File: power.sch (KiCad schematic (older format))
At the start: 44 parts, among them CON1 BARREL_JACK, J1 JMP, U2 WM8778-units, U3 AP3211, U4 AZ1117C, U5 TC1185

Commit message: ksch: add stuff that isn't on soldered prototype yet
this hopefully completes the rev. A schematics
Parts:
- C201: renamed from C1; footprint (none) -> Capacitors_SMD:C_0805_HandSoldering
- C202: renamed from C2; footprint (none) -> Capacitors_SMD:C_0805_HandSoldering
- C203: renamed from C3; footprint (none) -> Capacitors_SMD:C_0805_HandSoldering
- C204: renamed from C4; footprint (none) -> Capacitors_SMD:C_0805_HandSoldering
- C205: renamed from C5; footprint (none) -> Capacitors_SMD:C_0805_HandSoldering
- C206: renamed from C6; footprint (none) -> Capacitors_SMD:C_0805_HandSoldering
- C207: renamed from C7; footprint (none) -> Capacitors_SMD:C_0805_HandSoldering
- C208: renamed from C8; footprint (none) -> Capacitors_SMD:C_0805_HandSoldering
- C209: renamed from C9; footprint (none) -> Capacitors_SMD:C_0805_HandSoldering
- C210, C217, C219, C220, C221, C222, C226, C227, C228, C229, C230: renamed from C?; footprint (none) -> Capacitors_SMD:C_0805_HandSoldering
- C211: renamed from C10; footprint (none) -> Capacitors_SMD:C_0805_HandSoldering
- C212: renamed from C12; footprint (none) -> Capacitors_SMD:C_0805_HandSoldering
- C213: renamed from C13; footprint (none) -> Capacitors_SMD:C_0805_HandSoldering
- C214: renamed from C11; footprint (none) -> Capacitors_SMD:C_0805_HandSoldering
- C215: renamed from C14; footprint (none) -> Capacitors_SMD:C_0805_HandSoldering
- C216: renamed from C15; footprint (none) -> Capacitors_SMD:C_0805_HandSoldering
- C218: renamed from C16; footprint (none) -> Capacitors_SMD:C_0805_HandSoldering
- C223: renamed from C17; footprint (none) -> Capacitors_SMD:C_0805_HandSoldering
- C224: renamed from C18; footprint (none) -> Capacitors_SMD:C_0805_HandSoldering
- C225: renamed from C19; footprint (none) -> Capacitors_SMD:C_0805_HandSoldering
- CON201: renamed from CON1; footprint (none) -> Socket_Strips:Socket_Strip_Straight_1x02_Pitch2.54mm
- D201: renamed from D?; footprint (none) -> Diodes_THT:D_DO-35_SOD27_P7.62mm_Horizontal
- D202: renamed from D1; footprint (none) -> Diodes_THT:D_DO-35_SOD27_P7.62mm_Horizontal
- J201: renamed from J1; footprint (none) -> footprints:netconnector
- L201: renamed from L1; footprint (none) -> Resistors_Universal:Resistor_SMDuniversal_0805to1206_HandSoldering
- R201: renamed from R1; footprint (none) -> Resistors_THT:R_Axial_DIN0207_L6.3mm_D2.5mm_P7.62mm_Horizontal
- R202: renamed from R2; footprint (none) -> Resistors_THT:R_Axial_DIN0207_L6.3mm_D2.5mm_P7.62mm_Horizontal
- R203: renamed from R3; footprint (none) -> Resistors_THT:R_Axial_DIN0207_L6.3mm_D2.5mm_P7.62mm_Horizontal
- SW201: renamed from SW?; value SW_Push -> reset; footprint (none) -> Buttons_Switches_THT:SW_PUSH_6mm
- U201: renamed from U2; footprint (none) -> footprints:SSOP-28_5.3x10.2mm_Pitch0.65mm_HandSolder
- U202: renamed from U3; footprint (none) -> TO_SOT_Packages_SMD:SOT-23-6_Handsoldering
- U203: renamed from U4; footprint (none) -> footprints:SOT-223-3Lead_TabPin2_HandSoldering
- U204: renamed from U5; footprint (none) -> TO_SOT_Packages_SMD:SOT-23-5_HandSoldering
- U205: renamed from U?; footprint (none) -> footprints:LQFP-64_10x10mm_Pitch0.5mm_HandSolder
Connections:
- no-connect marks 1 -> 0

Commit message: ksch: reannotate schematics to have a single style of part-naming
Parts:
- renumbered C201 to C1, C210 to C10, C211 to C11, C212 to C12, C213 to C13, C214 to C14, C215 to C15, C216 to C16, C217 to C17, C218 to C18, C219 to C19, C202 to C2, C220 to C20, C221 to C21, C222 to C22, C223 to C23, C224 to C24, C225 to C25, C226 to C26, C227 to C27, C228 to C28, C229 to C29, C203 to C3, C230 to C30, C204 to C4, C205 to C5, C206 to C6, C207 to C7, C208 to C8, C209 to C9, CON201 to CON1, D201 to D1, D202 to D2, J201 to J1, L201 to L1, R201 to R1, R202 to R2, R203 to R3, SW201 to SW1, U201 to U1, U202 to U2, U203 to U3, U204 to U4, U205 to U5

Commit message: ksch: change power connector to DC5525
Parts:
- CON1: footprint Socket_Strips:Socket_Strip_Straight_1x02_Pitch2.54mm -> footprints:PJ-037A
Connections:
- wire segments 84 -> 86
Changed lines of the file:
@@
 LIBS:ftdi
 LIBS:gennum
-LIBS:graphic
 LIBS:hc11
 LIBS:intel
@@
 LIBS:leds
 LIBS:linear
-LIBS:logo
 LIBS:maxim
 LIBS:mechanical
@@
 F 0 "CON1" H 1350 1900 50  0000 C CNN
 F 1 "BARREL_JACK" H 1400 1500 50  0000 C CNN
-F 2 "Socket_Strips:Socket_Strip_Straight_1x02_Pitch2.54mm" H 1600 1650 50  0001 C CNN
+F 2 "footprints:PJ-037A" H 1600 1650 50  0001 C CNN
 F 3 "" H 1600 1650 50  0000 C CNN
 	1    1600 1650
@@
 Text GLabel 7650 5550 0    60   Input ~ 0
 BOOT
+Wire Wire Line
+	1900 1650 1950 1650
+Wire Wire Line
+	1950 1650 1950 1750
+Connection ~ 1950 1750
 $EndSCHEMATC

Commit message: k: fix pcb
power connector trouble
wrong footprint for caps
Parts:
- CON1: symbol BARREL_JACK -> BARREL_JACK_2P
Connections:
- wire segments 86 -> 84
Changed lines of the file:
@@
 $EndDescr
 $Comp
-L BARREL_JACK CON1
+L BARREL_JACK_2P CON1
 U 1 1 58B35157
 P 1600 1650
@@
 Text GLabel 7650 5550 0    60   Input ~ 0
 BOOT
-Wire Wire Line
-	1900 1650 1950 1650
-Wire Wire Line
-	1950 1650 1950 1750
-Connection ~ 1950 1750
 $EndSCHEMATC

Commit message: ksch: change component values to include the unit except for resistors add more info to some devices
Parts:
- C17: value 0.1u -> 100nF
- C19, C21, C26, C27, C28, C29: value 100n -> 100nF
- C2, C4, C5, C6, C7, C9: value 0.1uF -> 100nF
- C20: value 1u -> 1uF
- C22, C30: value 4.7u -> 4.7uF
- U2: value AP3211 -> AP3211KTR
- U3: value AZ1117C -> AZ1117CH-3.3
- U4: value TC1185 -> TC1185-5.0
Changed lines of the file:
@@
 Sheet 2 4
 Title "OpenLoop"
-Date "2017-09-25"
+Date "2017-10-02"
 Rev "A"
 Comp ""
@@
 P 4100 1750
 F 0 "U2" H 4000 2100 60  0000 C CNN
-F 1 "AP3211" H 4100 1450 60  0000 C CNN
+F 1 "AP3211KTR" H 4100 1450 60  0000 C CNN
 F 2 "TO_SOT_Packages_SMD:SOT-23-6_Handsoldering" H 4100 1750 60  0001 C CNN
 F 3 "" H 4100 1750 60  0000 C CNN
@@
 P 7600 1150
 F 0 "U3" H 7500 1350 60  0000 C CNN
-F 1 "AZ1117C" H 7600 950 60  0000 C CNN
+F 1 "AZ1117CH-3.3" H 7600 950 60  0000 C CNN
 F 2 "footprints:SOT-223-3Lead_TabPin2_HandSoldering" H 7600 1150 60  0001 C CNN
 F 3 "" H 7600 1150 60  0001 C CNN
@@
 P 7600 2600
 F 0 "U4" H 7500 2900 60  0000 C CNN
-F 1 "TC1185" H 7600 2300 60  0000 C CNN
+F 1 "TC1185-5.0" H 7600 2300 60  0000 C CNN
 F 2 "TO_SOT_Packages_SMD:SOT-23-5_HandSoldering" H 7600 2600 60  0001 C CNN
 F 3 "" H 7600 2600 60  0001 C CNN
@@
 P 2200 4800
 F 0 "C2" H 2210 4870 50  0000 L CNN
-F 1 "0.1uF" H 2210 4720 50  0000 L CNN
+F 1 "100nF" H 2210 4720 50  0000 L CNN
 F 2 "Capacitors_SMD:C_0805_HandSoldering" H 2200 4800 50  0001 C CNN
 F 3 "" H 2200 4800 50  0000 C CNN
@@
 P 4450 4150
 F 0 "C5" H 4460 4220 50  0000 L CNN
-F 1 "0.1uF" H 4460 4070 50  0000 L CNN
+F 1 "100nF" H 4460 4070 50  0000 L CNN
 F 2 "Capacitors_SMD:C_0805_HandSoldering" H 4450 4150 50  0001 C CNN
 F 3 "" H 4450 4150 50  0000 C CNN
@@
 P 4450 4650
 F 0 "C6" H 4460 4720 50  0000 L CNN
-F 1 "0.1uF" H 4460 4570 50  0000 L CNN
+F 1 "100nF" H 4460 4570 50  0000 L CNN
 F 2 "Capacitors_SMD:C_0805_HandSoldering" H 4450 4650 50  0001 C CNN
 F 3 "" H 4450 4650 50  0000 C CNN
@@
 P 4450 5150
 F 0 "C7" H 4460 5220 50  0000 L CNN
-F 1 "0.1uF" H 4460 5070 50  0000 L CNN
+F 1 "100nF" H 4460 5070 50  0000 L CNN
 F 2 "Capacitors_SMD:C_0805_HandSoldering" H 4450 5150 50  0001 C CNN
 F 3 "" H 4450 5150 50  0000 C CNN
@@
 P 4400 5750
 F 0 "C4" H 4410 5820 50  0000 L CNN
-F 1 "0.1uF" H 4410 5670 50  0000 L CNN
+F 1 "100nF" H 4410 5670 50  0000 L CNN
 F 2 "Capacitors_SMD:C_0805_HandSoldering" H 4400 5750 50  0001 C CNN
 F 3 "" H 4400 5750 50  0000 C CNN
@@
 P 4600 5600
 F 0 "C9" H 4610 5670 50  0000 L CNN
-F 1 "0.1uF" H 4610 5520 50  0000 L CNN
+F 1 "100nF" H 4610 5520 50  0000 L CNN
 F 2 "Capacitors_SMD:C_0805_HandSoldering" H 4600 5600 50  0001 C CNN
 F 3 "" H 4600 5600 50  0000 C CNN
@@
 P 7000 4700
 F 0 "C17" H 7010 4770 50  0000 L CNN
-F 1 "0.1u" H 7010 4620 50  0000 L CNN
+F 1 "100nF" H 7010 4620 50  0000 L CNN
 F 2 "Capacitors_SMD:C_0805_HandSoldering" H 7000 4700 50  0001 C CNN
 F 3 "" H 7000 4700 50  0001 C CNN
@@
 P 7450 5850
 F 0 "C22" H 7460 5920 50  0000 L CNN
-F 1 "4.7u" H 7460 5770 50  0000 L CNN
+F 1 "4.7uF" H 7460 5770 50  0000 L CNN
 F 2 "Capacitors_SMD:C_0805_HandSoldering" H 7450 5850 50  0001 C CNN
 F 3 "" H 7450 5850 50  0001 C CNN
@@
 P 9400 5850
 F 0 "C29" H 9410 5920 50  0000 L CNN
-F 1 "100n" H 9410 5770 50  0000 L CNN
+F 1 "100nF" H 9410 5770 50  0000 L CNN
 F 2 "Capacitors_SMD:C_0805_HandSoldering" H 9400 5850 50  0001 C CNN
 F 3 "" H 9400 5850 50  0001 C CNN
@@
 P 9400 5350
 F 0 "C28" H 9410 5420 50  0000 L CNN
-F 1 "100n" H 9410 5270 50  0000 L CNN
+F 1 "100nF" H 9410 5270 50  0000 L CNN
 F 2 "Capacitors_SMD:C_0805_HandSoldering" H 9400 5350 50  0001 C CNN
 F 3 "" H 9400 5350 50  0001 C CNN
@@
 P 9400 4850
 F 0 "C27" H 9410 4920 50  0000 L CNN
-F 1 "100n" H 9410 4770 50  0000 L CNN
+F 1 "100nF" H 9410 4770 50  0000 L CNN
 F 2 "Capacitors_SMD:C_0805_HandSoldering" H 9400 4850 50  0001 C CNN
 F 3 "" H 9400 4850 50  0001 C CNN
@@
 P 9400 4350
 F 0 "C26" H 9410 4420 50  0000 L CNN
-F 1 "100n" H 9410 4270 50  0000 L CNN
+F 1 "100nF" H 9410 4270 50  0000 L CNN
 F 2 "Capacitors_SMD:C_0805_HandSoldering" H 9400 4350 50  0001 C CNN
 F 3 "" H 9400 4350 50  0001 C CNN
@@
 P 7450 5100
 F 0 "C21" H 7460 5170 50  0000 L CNN
-F 1 "100n" H 7460 5020 50  0000 L CNN
+F 1 "100nF" H 7460 5020 50  0000 L CNN
 F 2 "Capacitors_SMD:C_0805_HandSoldering" H 7450 5100 50  0001 C CNN
 F 3 "" H 7450 5100 50  0001 C CNN
@@
 P 7200 5100
 F 0 "C20" H 7210 5170 50  0000 L CNN
-F 1 "1u" H 7210 5020 50  0000 L CNN
+F 1 "1uF" H 7210 5020 50  0000 L CNN
 F 2 "Capacitors_SMD:C_0805_HandSoldering" H 7200 5100 50  0001 C CNN
 F 3 "" H 7200 5100 50  0001 C CNN
@@
 P 9800 5050
 F 0 "C30" H 9810 5120 50  0000 L CNN
-F 1 "4.7u" H 9810 4970 50  0000 L CNN
+F 1 "4.7uF" H 9810 4970 50  0000 L CNN
 F 2 "Capacitors_SMD:C_0805_HandSoldering" H 9800 5050 50  0001 C CNN
 F 3 "" H 9800 5050 50  0001 C CNN
@@
 P 7100 4200
 F 0 "C19" H 7110 4270 50  0000 L CNN
-F 1 "100n" H 7110 4120 50  0000 L CNN
+F 1 "100nF" H 7110 4120 50  0000 L CNN
 F 2 "Capacitors_SMD:C_0805_HandSoldering" H 7100 4200 50  0001 C CNN
 F 3 "" H 7100 4200 50  0001 C CNN

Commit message: migrate to kicad v5
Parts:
- C1, C10, C11, C12, C13, C14, C15, C16, C18, C19, C2, C21, C22, C23, C24, C25, C26, C27, C28, C29, C3, C4, C5, C6, C7, C8, C9: symbol C_Small -> Device:C_Small
- C17, C20, C30: symbol C -> Device:C
- CON1: symbol BARREL_JACK_2P -> openloop:BARREL_JACK_2P
- D1: symbol D_Small_ALT -> Device:D_Small_ALT
- D2: symbol D_Schottky_Small_ALT -> Device:D_Schottky_Small_ALT
- J1: symbol JMP -> openloop:JMP
- L1: symbol L_Small -> Device:L_Small
- R1, R2, R3: symbol R_Small -> Device:R_Small
- SW1: symbol SW_Push -> Switch:SW_Push
- U1: symbol WM8778-units -> openloop:WM8778-units
- U2: symbol AP3211 -> openloop:AP3211
- U3: symbol AZ1117C -> openloop:AZ1117C
- U4: symbol TC1185 -> openloop:TC1185
- U5: symbol STM32F401RC -> openloop:STM32F401RC
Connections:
- wire segments 84 -> 126

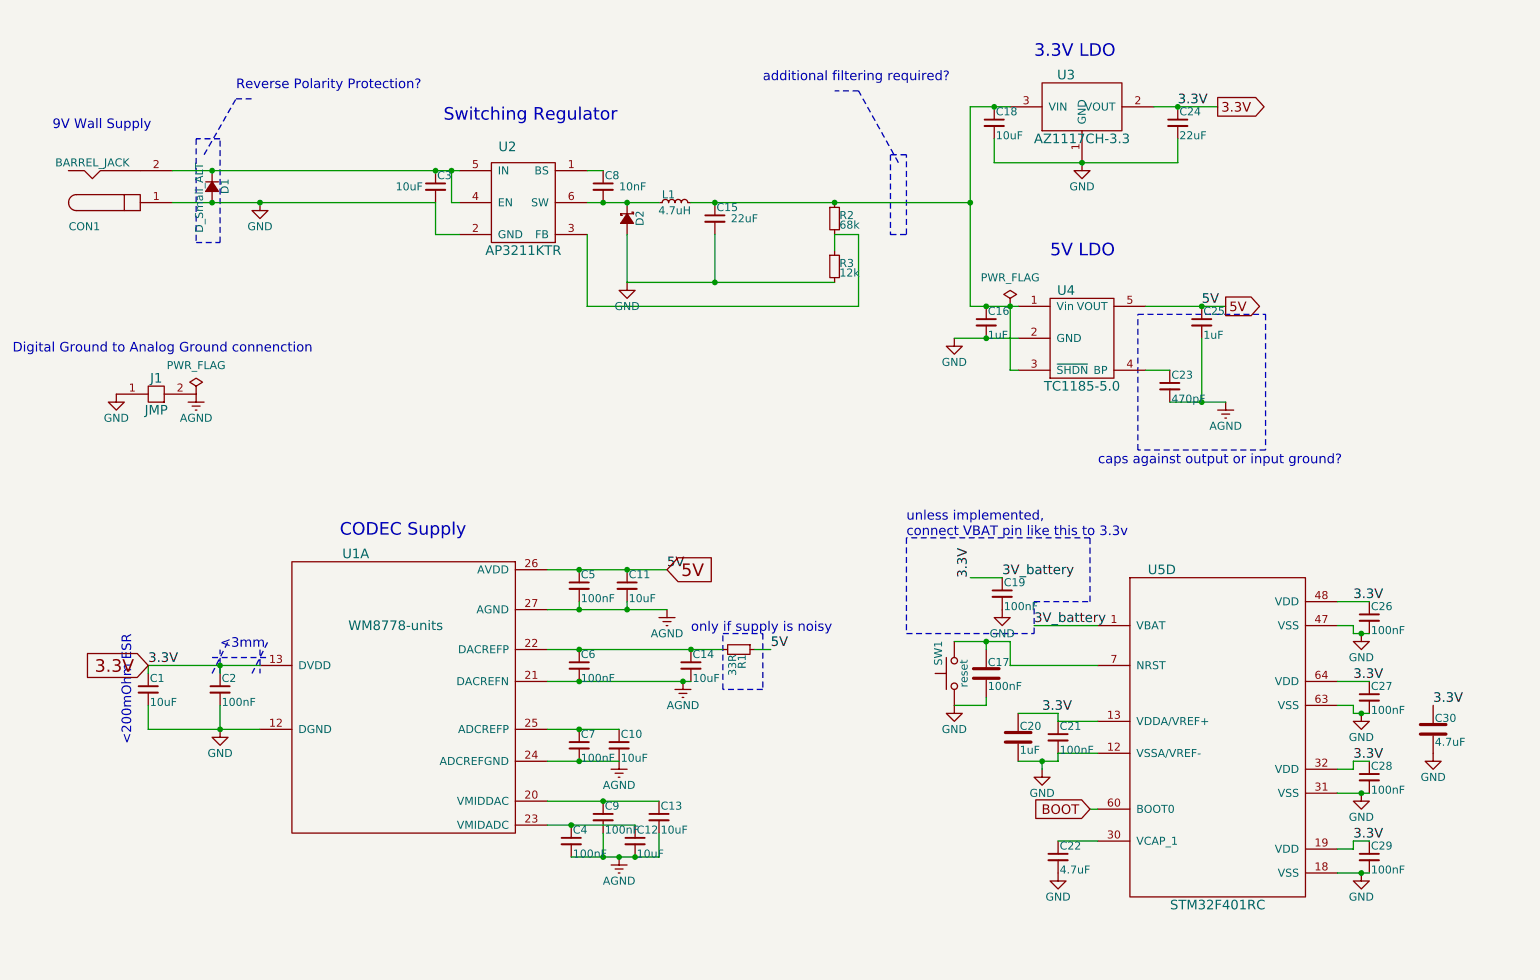
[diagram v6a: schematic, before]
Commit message: ready for print
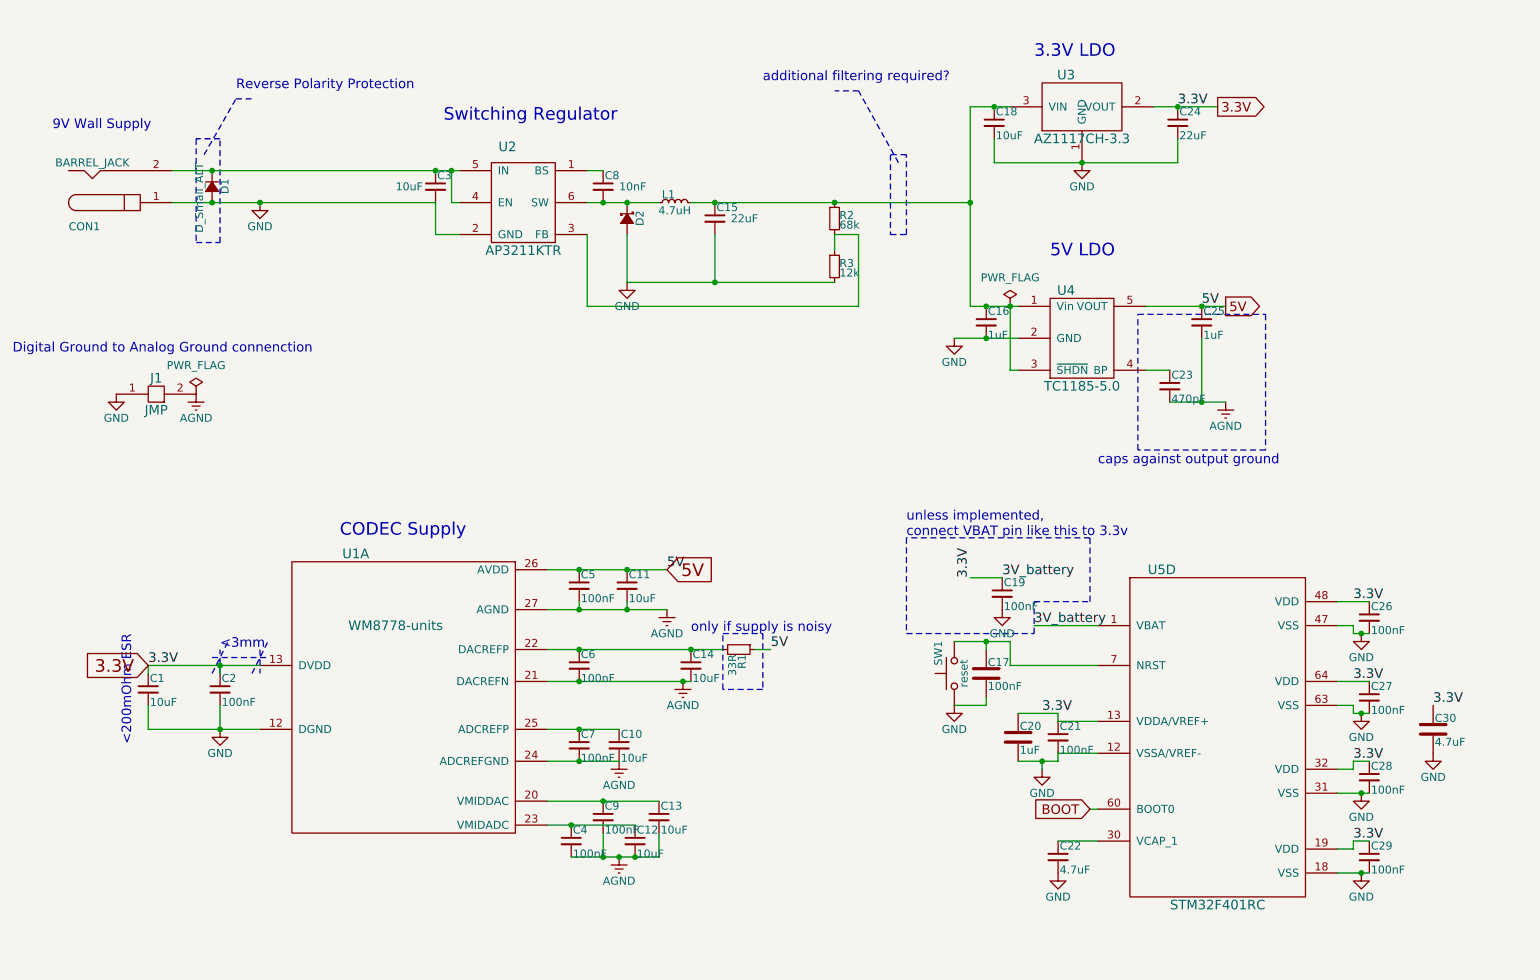
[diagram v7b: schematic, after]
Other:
- note added: "Reverse Polarity Protection"
- note added: "caps against output ground"
- note removed: "Reverse Polarity Protection?"
- note removed: "caps against output or input ground?"
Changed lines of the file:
@@
 Sheet 2 4
 Title "OpenLoop"
-Date "2017-10-02"
+Date "2018-06-20"
 Rev "A"
 Comp ""
@@
 9V Wall Supply
 Text Notes 2300 1050 0    60   ~ 0
-Reverse Polarity Protection?
+Reverse Polarity Protection
 Text Notes 5600 1000 0    60   ~ 0
 additional filtering required?
@@
 3.3V
 Text Notes 7700 3400 0    60   ~ 0
-caps against output or input ground?
+caps against output ground
 $Comp
 L openloop:AGND #PWR09
